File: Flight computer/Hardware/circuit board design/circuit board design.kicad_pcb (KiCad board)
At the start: 4 copper layers, 30.5 x 82.6 mm, 90 parts, among them J1 Conn_01x05, J2 USB_B_Micro, J3 Screw_Terminal_01x06, J4 Conn_01x02, J5 Screw_Terminal_01x06, J6 Conn_Coaxial, J7 Conn_Coaxial, U1 IIS2MDC, U10 BMI088, U11 ATSAML21J18B-AUT, U14 MAX40200AUK, U15 LD3985G33R_TSOT23, U2 0433BM41A0019E, U3 Si4463, U4 MAX-M8C, U5 Si7232DN, U6 Si7232DN, U7 W74M64FV, U8 MS5607-02BA, U9 STF202-22T1G, X1 TM-32.000-AF3-33-S-Oscillator, Y3 16MHz

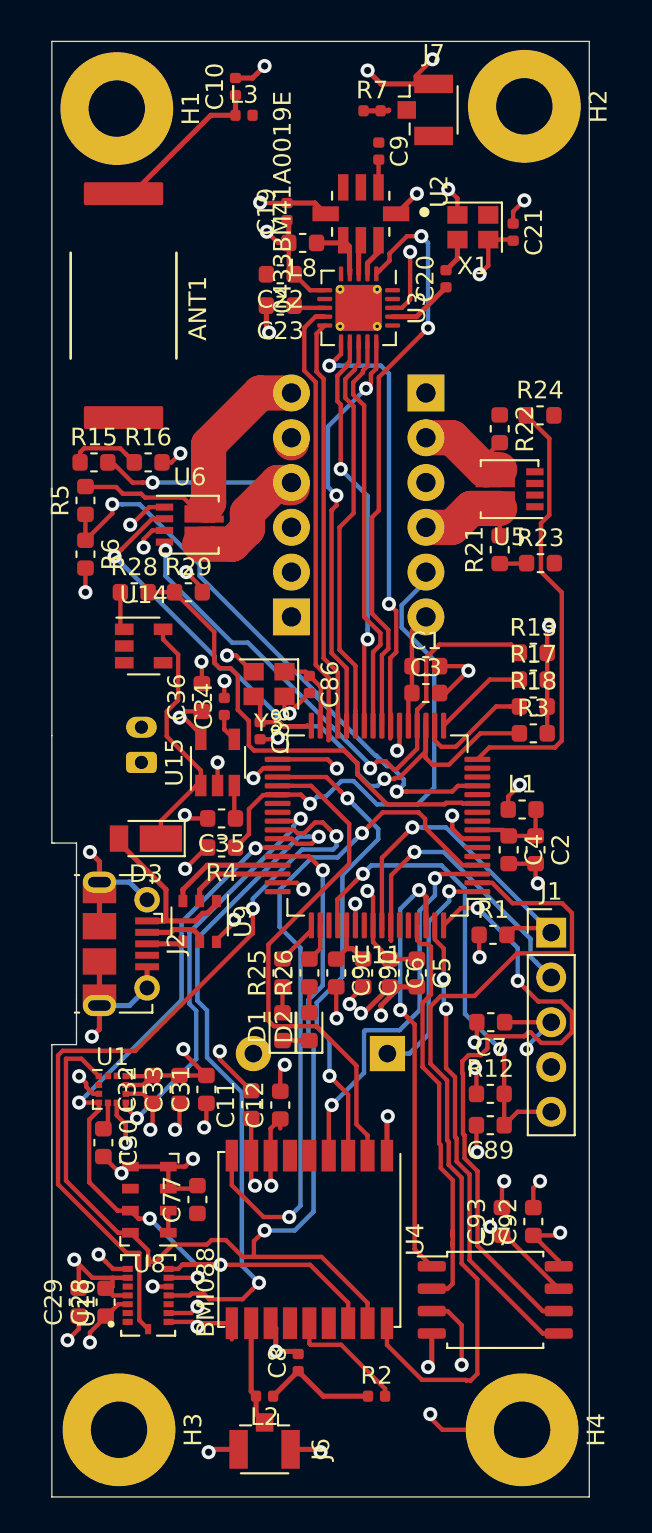
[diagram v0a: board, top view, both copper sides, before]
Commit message: only 2 or 3 connections left to route
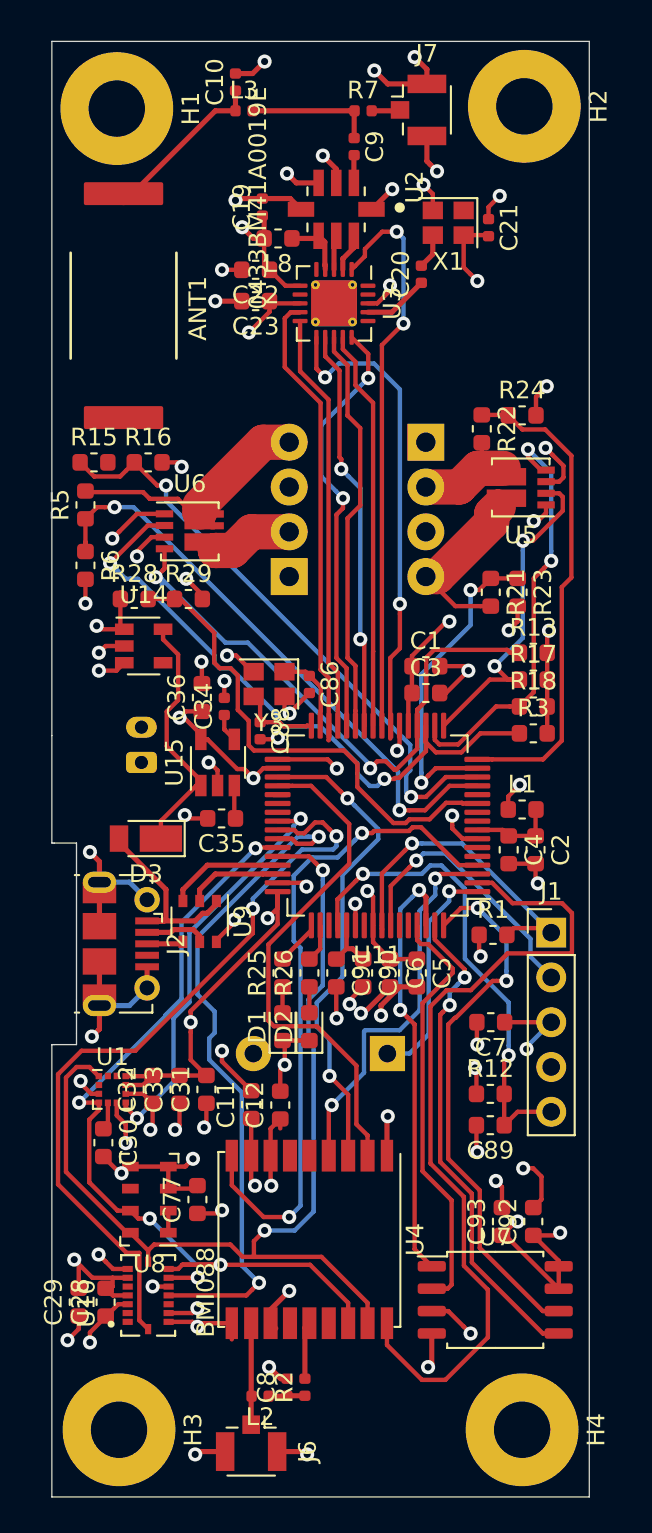
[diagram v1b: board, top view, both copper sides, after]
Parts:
- removed R4: 1K, Resistor_SMD:R_0603_1608Metric
- J3, J5: value Screw_Terminal_01x06 -> Screw_Terminal_01x04; footprint flight-computer:TerminalBlock_TE_282834-6_1x06_P2.54mm_Horizontal -> flight-computer:TerminalBlock_TE_282834-4_1x04_P2.54mm_Horizontal
- moved R2 4.10 mm to (265.8, 322.7), turned to 90 degrees
- moved J5 2.79 mm to (272.7, 269.1)
- moved R21 2.47 mm to (276.4, 277.6), turned to 270 degrees
- moved J3 2.29 mm to (264.9, 276.7)
- moved R23 2.10 mm to (277.9, 277.6), turned to 270 degrees
- moved C8 1.53 mm to (264.8, 322.7)
- moved L8 1.42 mm to (264.3, 257.6)
- moved C22 1.42 mm to (263.0, 259.3)
- moved C9 1.42 mm to (268.6, 252.3)
- moved U3 1.42 mm to (267.5, 261.2)
- moved X1 1.42 mm to (273.9, 256.7)
- moved C19 1.42 mm to (263.4, 255.8)
- moved U2 1.42 mm to (267.6, 255.9)
- moved C20 1.42 mm to (272.4, 259.6)
- moved C21 1.42 mm to (276.2, 256.9)
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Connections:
- J3 pad 1: Net-(J3-Pad1) -> Vdrive
- J3 pad 2: Vdrive -> /pyro_driver/FET_B
- J3 pad 3: Net-(J3-Pad1) -> Vdrive
- J3 pad 4: /pyro_driver/FET_B -> /pyro_driver/FET_A
- J5 pad 1: Net-(J3-Pad1) -> Vdrive
- J5 pad 3: Net-(J3-Pad1) -> Vdrive
- U11 pad 37: /MCU/ARMED -> (no net)
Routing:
- net +3V3: track 82.5 -> 257.7 mm, vias 21 -> 25
- net /MCU/MCU_PA05: track 4.07 -> 33.9 mm, vias 0 -> 2
- net /MCU/ARMED: track 28.8 -> 0.00 mm, vias 1 -> 0
- net Vdrive: track 24.7 -> 5.46 mm, vias 0 -> 2
- net /pyro_driver/FIRE_D: track 6.73 -> 24.2 mm, vias 0 -> 2
- net /MCU/MCU_PA06: track 1.53 -> 18.5 mm, vias 0 -> 2
- net /pyro_driver/FIRE_C: track 5.38 -> 19.7 mm, vias 0 -> 2
- net /pyro_driver/FET_B: track 18.7 -> 4.94 mm, vias 1 -> 0
- net GND: track 150.9 -> 163.8 mm, vias 58 -> 66
- net Net-(C9-Pad1): track 0.00 -> 7.17 mm
- net /MCU/MCU_SCLK4: track 37.1 -> 30.9 mm
- net Net-(C8-Pad1): track 6.56 -> 2.10 mm
- net /pyro_driver/FET_C: track 6.66 -> 10.4 mm
- net Net-(R2-Pad2): track 6.93 -> 3.25 mm
- net /pyro_driver/FET_A: track 16.6 -> 13.7 mm
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- added copper zone on VCC.Cu, net Vdrive
- removed copper zone on VCC.Cu, net +3V3
